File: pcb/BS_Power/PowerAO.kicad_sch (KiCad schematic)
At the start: 27 parts, among them IC1 TPS51396ARJER

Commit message: Before 5V regulator replacement
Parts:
- IC1: LCSC Part (none) -> C3192016
- L1: LCSC Part (none) -> C2761915
- L2: LCSC Part (none) -> C844980
- PS2: LCSC Part (none) -> C122479
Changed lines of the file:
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@@
+      (effects (font (size 1.27 1.27)) hide)
+    )
+    (property "LCSC Part" "C2761915" (id 4) (at 124.46 29.21 0)
       (effects (font (size 1.27 1.27)) hide)
     )
@@
     (property "Manufacturer_Part_Number" "TPS51396ARJER" (id 9) (at 101.6 57.15 0)
       (effects (font (size 1.27 1.27)) (justify left) hide)
+    )
+    (property "LCSC Part" "C3192016" (id 10) (at 74.93 41.91 0)
+      (effects (font (size 1.27 1.27)) hide)
     )
     (pin "1")
@@
       (effects (font (size 1.27 1.27)) (justify left) hide)
     )
+    (property "LCSC Part" "C122479" (id 10) (at 90.17 115.57 0)
+      (effects (font (size 1.27 1.27)) hide)
+    )
     (pin "1")
     (pin "10")
@@
       (effects (font (size 1.27 1.27)) hide)
     )
+    (property "LCSC Part" "C844980" (id 4) (at 113.03 101.6 90)
+      (effects (font (size 1.27 1.27)) hide)
+    )

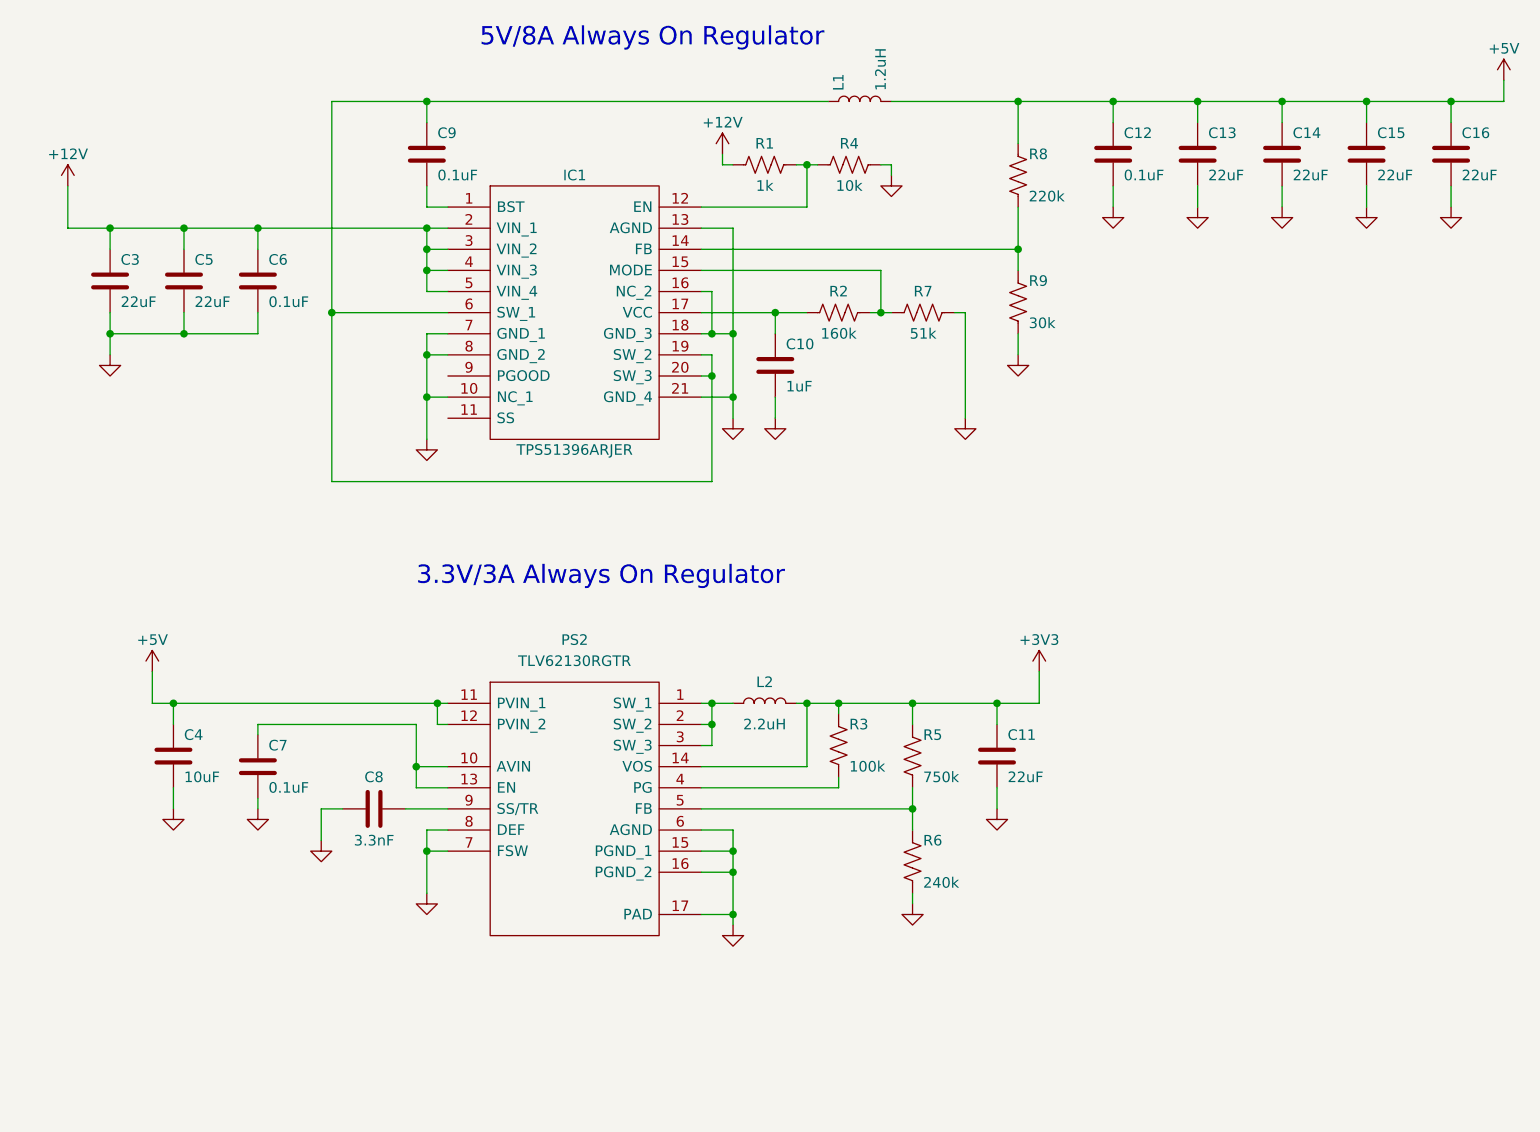
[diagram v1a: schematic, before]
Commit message: BS_Power updates
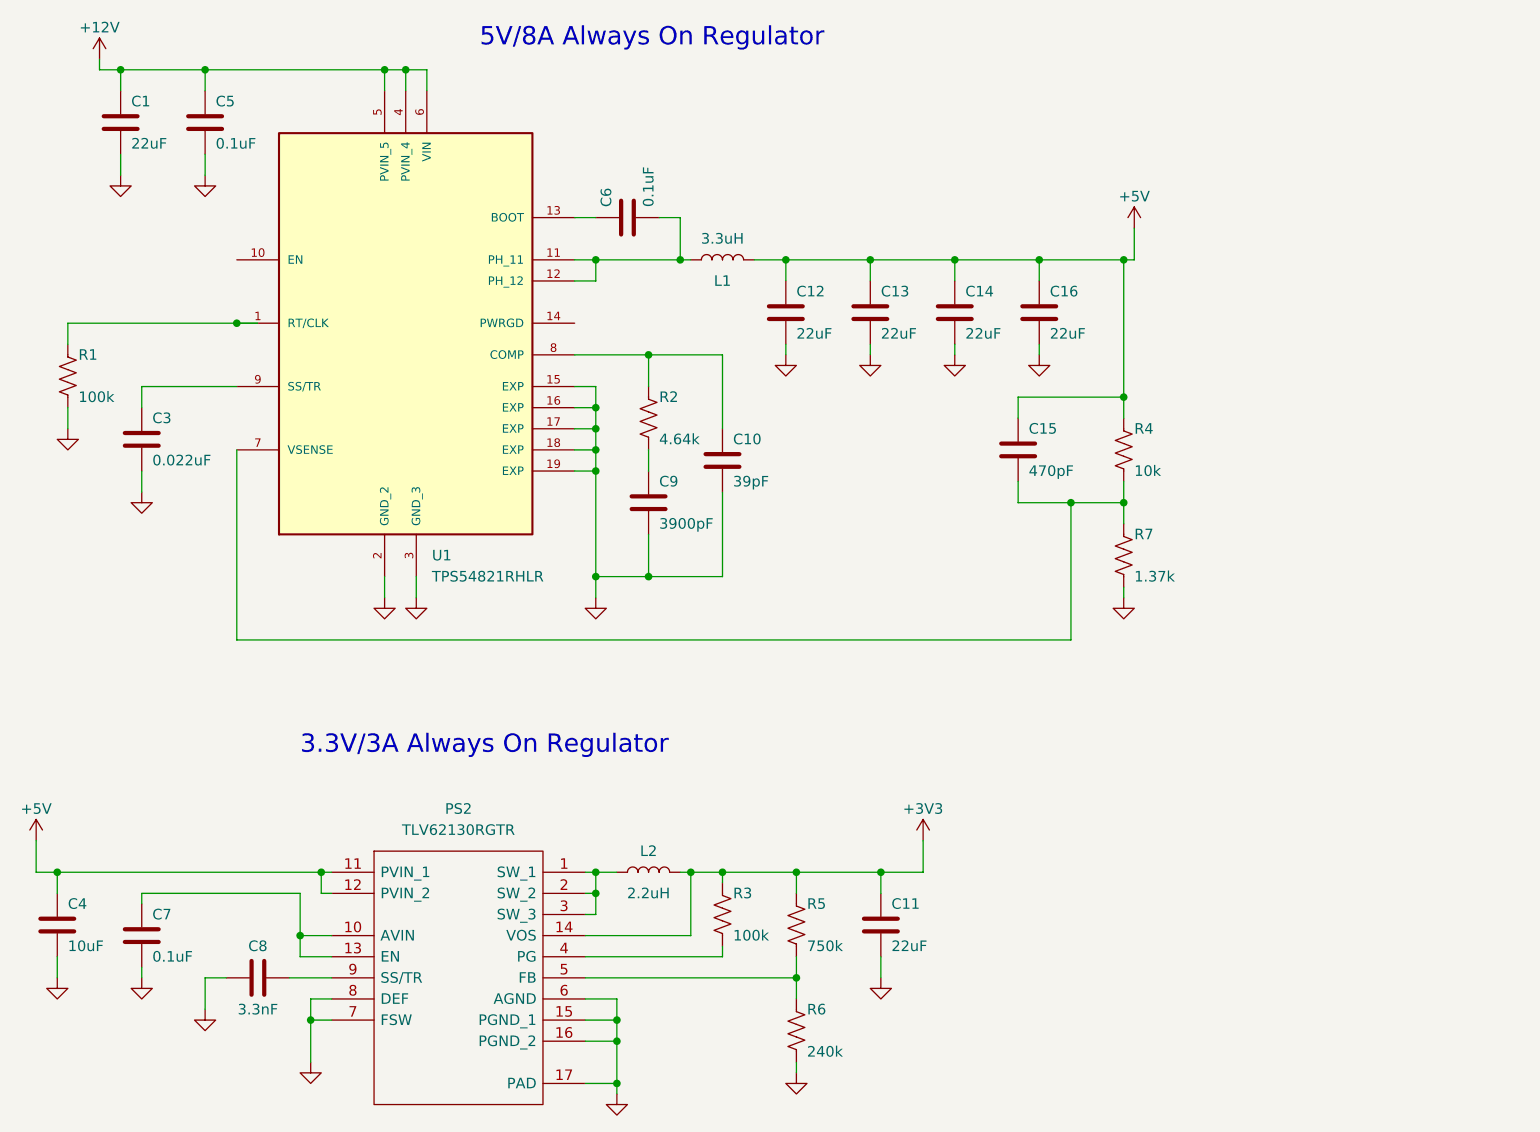
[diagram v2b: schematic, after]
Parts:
- removed IC1: TPS51396ARJER, SamacSys_Parts:TPS51396ARJER, symbol SamacSys_Parts:TPS51396ARJER
- removed R8: 220k, Resistor_SMD:R_0603_1608Metric, symbol Device:R_US
- removed R9: 30k, Resistor_SMD:R_0603_1608Metric, symbol Device:R_US
- added C1: 22uF, Capacitor_SMD:C_0805_2012Metric, symbol Device:C
- added U1: TPS54821RHLR, Parts:IC_TPS54821RHLR, symbol TPS54821RHLR:TPS54821RHLR
- C10: value 1uF -> 39pF
- C12: value 0.1uF -> 22uF; footprint Capacitor_SMD:C_0603_1608Metric -> Capacitor_SMD:C_0805_2012Metric
- C15: value 22uF -> 470pF; footprint Capacitor_SMD:C_0805_2012Metric -> Capacitor_SMD:C_0603_1608Metric
- C3: value 22uF -> 0.022uF; footprint Capacitor_SMD:C_0805_2012Metric -> Capacitor_SMD:C_0603_1608Metric
- C5: value 22uF -> 0.1uF; footprint Capacitor_SMD:C_0805_2012Metric -> Capacitor_SMD:C_0603_1608Metric
- C9: value 0.1uF -> 3900pF
- L1: value 1.2uH -> 3.3uH; footprint Beefy:L_10.2x10.5 -> Beefy:L_6.7x7; LCSC Part C2761915 -> C2761959
- L2: footprint Beefy:L_4.45x4.06 -> Beefy:L_4.1x4.5; LCSC Part C844980 -> C2847469
- R1: value 1k -> 100k
- R2: value 160k -> 4.64k; footprint Resistor_SMD:R_0603_1608Metric -> Resistor_SMD:R_0402_1005Metric; LCSC Part (none) -> C60154
- R4: footprint Resistor_SMD:R_0603_1608Metric -> Resistor_SMD:R_0402_1005Metric; LCSC Part (none) -> C852428
- R7: value 51k -> 1.37k; footprint Resistor_SMD:R_0603_1608Metric -> Resistor_SMD:R_0402_1005Metric; LCSC Part (none) -> C705664
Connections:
- net +12V: now also C1.1, U1.4 (PVIN_4), U1.5 (PVIN_5), U1.6 (VIN); no longer C3.1, C6.1, R1.1
- net +5V: now also R4.1
- net GND: now also C9.2, R1.2, R7.2, C1.2, U1.15 (EXP), U1.16 (EXP), U1.17 (EXP), U1.18 (EXP), U1.19 (EXP), U1.2 (GND_2), U1.3 (GND_3); no longer C15.2, C6.2, R4.2, R7.1
- net at R2.2: now also C9.1; no longer R7.2
- net at L1.1: now also C6.2, U1.11 (PH_11), U1.12 (PH_12); no longer C9.1
- net at C10.1, R2.1: now also U1.8 (COMP)
- new net: R1.1, U1.1 (RT/CLK)
- new net: C6.1, U1.13 (BOOT)
- new net: C15.2, R4.2, R7.1, U1.7 (VSENSE)
- new net: C3.1, U1.9 (SS/TR)
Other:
- moved on the sheet: C11, C4, C7, C8, L2, PS2, R3, R5, R6
